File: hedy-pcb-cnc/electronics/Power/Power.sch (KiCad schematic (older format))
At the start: 11 parts

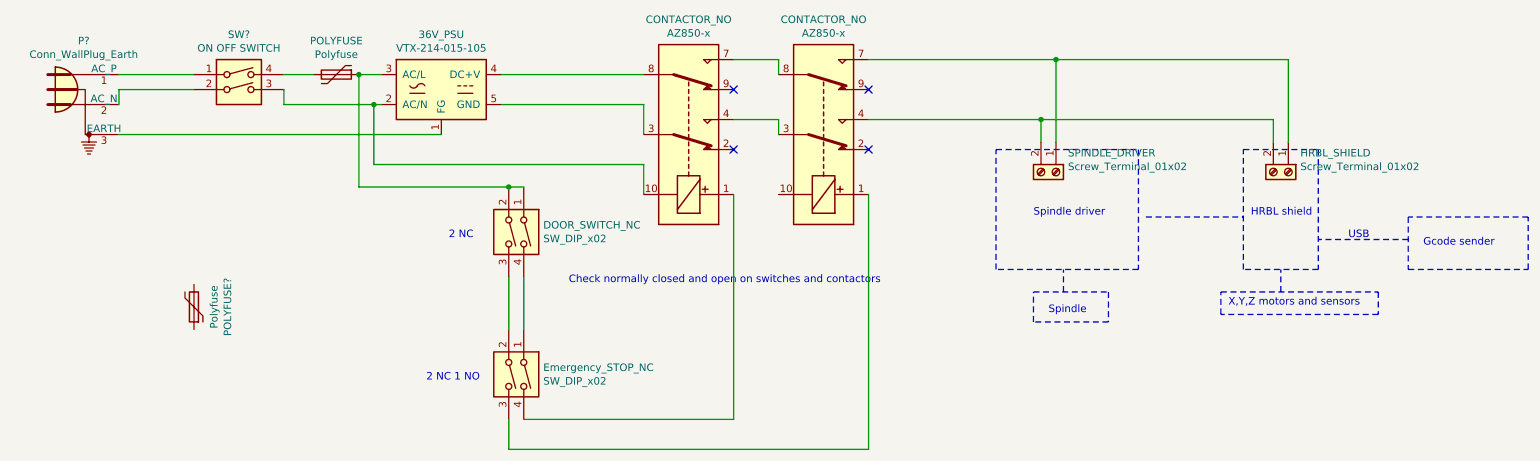
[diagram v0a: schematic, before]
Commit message: electronics
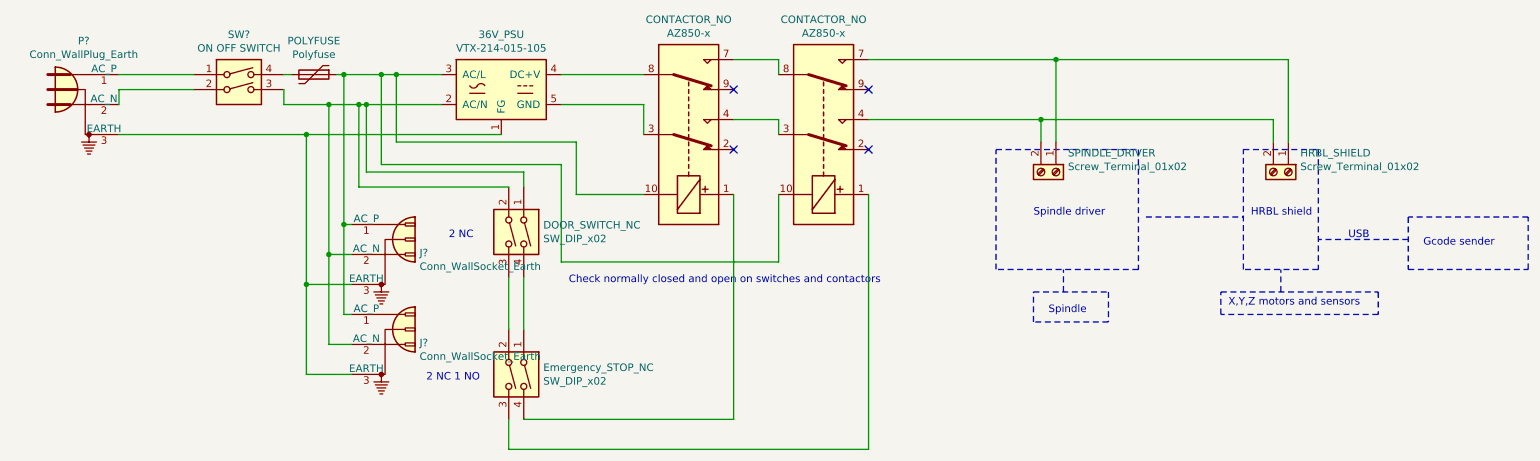
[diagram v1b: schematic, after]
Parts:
- removed POLYFUSE?: Polyfuse, symbol Device:Polyfuse
- added J? (x2): Conn_WallSocket_Earth, symbol Connector:Conn_WallSocket_Earth
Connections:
- net at 36V_PSU.2 (AC/N), SW?.3: now also DOOR_SWITCH_NC.1, DOOR_SWITCH_NC.2, J?.2 (AC_N), J?.2 (AC_N); no longer CONTACTOR_NO.10
- net at 36V_PSU.3 (AC/L), POLYFUSE.1: now also CONTACTOR_NO.10, CONTACTOR_NO.10, J?.1 (AC_P), J?.1 (AC_P); no longer DOOR_SWITCH_NC.1, DOOR_SWITCH_NC.2
- net at 36V_PSU.1 (FG), P?.3 (EARTH): now also J?.3 (EARTH), J?.3 (EARTH)
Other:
- moved on the sheet: 36V_PSU, POLYFUSE
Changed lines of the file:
@@
 	1    0    0    -1
 $EndComp
-$Comp
-L Device:Polyfuse POLYFUSE
-U 1 1 5B9A9611
-P 2850 1750
-F 0 "POLYFUSE" V 2625 1750 50  0000 C CNN
-F 1 "Polyfuse" V 2716 1750 50  0000 C CNN
-F 2 "" H 2900 1550 50  0001 L CNN
-F 3 "~" H 2850 1750 50  0001 C CNN
-	1    2850 1750
-	0    1    1    0
-$EndComp
-Wire Wire Line
-	2500 1750 2700 1750
 Wire Wire Line
 	2500 1850 2500 1950
@@
 L Converter_ACDC:VTX-214-015-105 36V_PSU
 U 1 1 5B9ABC32
-P 3550 1850
-F 0 "36V_PSU" H 3550 2217 50  0000 C CNN
-F 1 "VTX-214-015-105" H 3550 2126 50  0000 C CNN
-F 2 "Converter_ACDC:Converter_ACDC_Vigortronix_VTX-214-015-1xx_THT" H 3550 2200 50  0001 C CNN
-F 3 "http://www.vigortronix.com/15WattSMPSPCBModuleAC-DC" H 4650 1050 50  0001 C CNN
-	1    3550 1850
-	1    0    0    -1
-$EndComp
-Wire Wire Line
-	1400 2150 3550 2150
+P 3950 1850
+F 0 "36V_PSU" H 3950 2217 50  0000 C CNN
+F 1 "VTX-214-015-105" H 3950 2126 50  0000 C CNN
+F 2 "Converter_ACDC:Converter_ACDC_Vigortronix_VTX-214-015-1xx_THT" H 3950 2200 50  0001 C CNN
+F 3 "http://www.vigortronix.com/15WattSMPSPCBModuleAC-DC" H 5050 1050 50  0001 C CNN
+	1    3950 1850
+	1    0    0    -1
+$EndComp
+Wire Wire Line
+	1400 2150 2650 2150
 Wire Wire Line
 	4900 1950 4900 2150
-Wire Wire Line
-	3950 1950 4900 1950
 Wire Wire Line
 	4100 4050 5500 4050
@@
 2 NC
 Wire Wire Line
-	3950 1750 4900 1750
-Wire Wire Line
-	4000 2500 4100 2500
-Connection ~ 4000 2500
-Wire Wire Line
-	4900 2350 4900 2550
-Wire Wire Line
-	3000 1750 3150 1750
-Wire Wire Line
-	2500 1950 3100 1950
-Wire Wire Line
-	3000 1750 3000 2500
+	2500 1950 2800 1950
 Wire Wire Line
 	3000 2500 4000 2500
-Connection ~ 3000 1750
-Wire Wire Line
-	3100 1950 3100 2350
-Wire Wire Line
-	3100 2350 4900 2350
-Connection ~ 3100 1950
-Wire Wire Line
-	3100 1950 3150 1950
-$Comp
-L Device:Polyfuse POLYFUSE?
-U 1 1 5B9B9214
-P 1900 3300
-F 0 "POLYFUSE?" V 1675 3300 50  0000 C CNN
-F 1 "Polyfuse" V 1766 3300 50  0000 C CNN
-F 2 "" H 1950 3100 50  0001 L CNN
-F 3 "~" H 1900 3300 50  0001 C CNN
-	1    1900 3300
-	-1   0    0    1
-$EndComp
+$Comp
+L Device:Polyfuse POLYFUSE
+U 1 1 5B9A9611
+P 2700 1750
+F 0 "POLYFUSE" V 2475 1750 50  0000 C CNN
+F 1 "Polyfuse" V 2566 1750 50  0000 C CNN
+F 2 "" H 2750 1550 50  0001 L CNN
+F 3 "~" H 2700 1750 50  0001 C CNN
+	1    2700 1750
+	0    1    1    0
+$EndComp
+Wire Wire Line
+	2550 1750 2500 1750
+Wire Wire Line
+	2850 1750 2900 1750
+$Comp
+L Connector:Conn_WallSocket_Earth J?
+U 1 1 5BA52863
+P 3150 2950
+F 0 "J?" H 3405 2961 50  0000 L CNN
+F 1 "Conn_WallSocket_Earth" H 3405 2870 50  0000 L CNN
+F 2 "" H 2850 3050 50  0001 C CNN
+F 3 "~" H 2850 3050 50  0001 C CNN
+	1    3150 2950
+	1    0    0    -1
+$EndComp
+Wire Wire Line
+	2950 2750 2900 2750
+Wire Wire Line
+	2900 2750 2900 1750
+Connection ~ 2900 1750
+Wire Wire Line
+	2950 2950 2800 2950
+Wire Wire Line
+	2800 2950 2800 1950
+Connection ~ 2800 1950
+Wire Wire Line
+	2950 3150 2650 3150
+Wire Wire Line
+	2650 3150 2650 2150
+Connection ~ 2650 2150
+$Comp
+L Connector:Conn_WallSocket_Earth J?
+U 1 1 5BA54EE7
+P 3150 3550
+F 0 "J?" H 3405 3561 50  0000 L CNN
+F 1 "Conn_WallSocket_Earth" H 3405 3470 50  0000 L CNN
+F 2 "" H 2850 3650 50  0001 C CNN
+F 3 "~" H 2850 3650 50  0001 C CNN
+	1    3150 3550
+	1    0    0    -1
+$EndComp
+Wire Wire Line
+	2900 2750 2900 3350
+Wire Wire Line
+	2900 3350 2950 3350
+Connection ~ 2900 2750
+Wire Wire Line
+	2800 2950 2800 3550
+Wire Wire Line
+	2800 3550 2950 3550
+Connection ~ 2800 2950
+Wire Wire Line
+	2650 3150 2650 3750
+Wire Wire Line
+	2650 3750 2950 3750
+Connection ~ 2650 3150
+Wire Wire Line
+	2800 1950 3000 1950
+Wire Wire Line
+	3000 2500 3000 1950
+Connection ~ 3000 1950
+Wire Wire Line
+	4350 1750 4900 1750
+Wire Wire Line
+	4900 1950 4350 1950
+Wire Wire Line
+	2650 2150 3950 2150
+Wire Wire Line
+	3000 1950 3050 1950
+Wire Wire Line
+	4350 2350 4350 3000
+Wire Wire Line
+	4350 3000 5800 3000
+Wire Wire Line
+	5800 3000 5800 2550
+Wire Wire Line
+	4900 2550 4450 2550
+Wire Wire Line
+	4450 2550 4450 2200
+Wire Wire Line
+	4450 2200 3250 2200
+Wire Wire Line
+	3250 2200 3250 1750
+Connection ~ 3250 1750
+Wire Wire Line
+	3250 1750 3550 1750
+Wire Wire Line
+	2900 1750 3150 1750
+Wire Wire Line
+	3150 1750 3150 2350
+Connection ~ 3150 1750
+Wire Wire Line
+	3150 1750 3250 1750
+Wire Wire Line
+	3150 2350 4350 2350
+Wire Wire Line
+	4100 2500 4100 2400
+Wire Wire Line
+	4100 2400 3050 2400
+Wire Wire Line
+	3050 2400 3050 1950
+Connection ~ 3050 1950
+Wire Wire Line
+	3050 1950 3550 1950
 $EndSCHEMATC
